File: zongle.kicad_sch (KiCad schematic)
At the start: 20 parts, among them U1 453-00059R

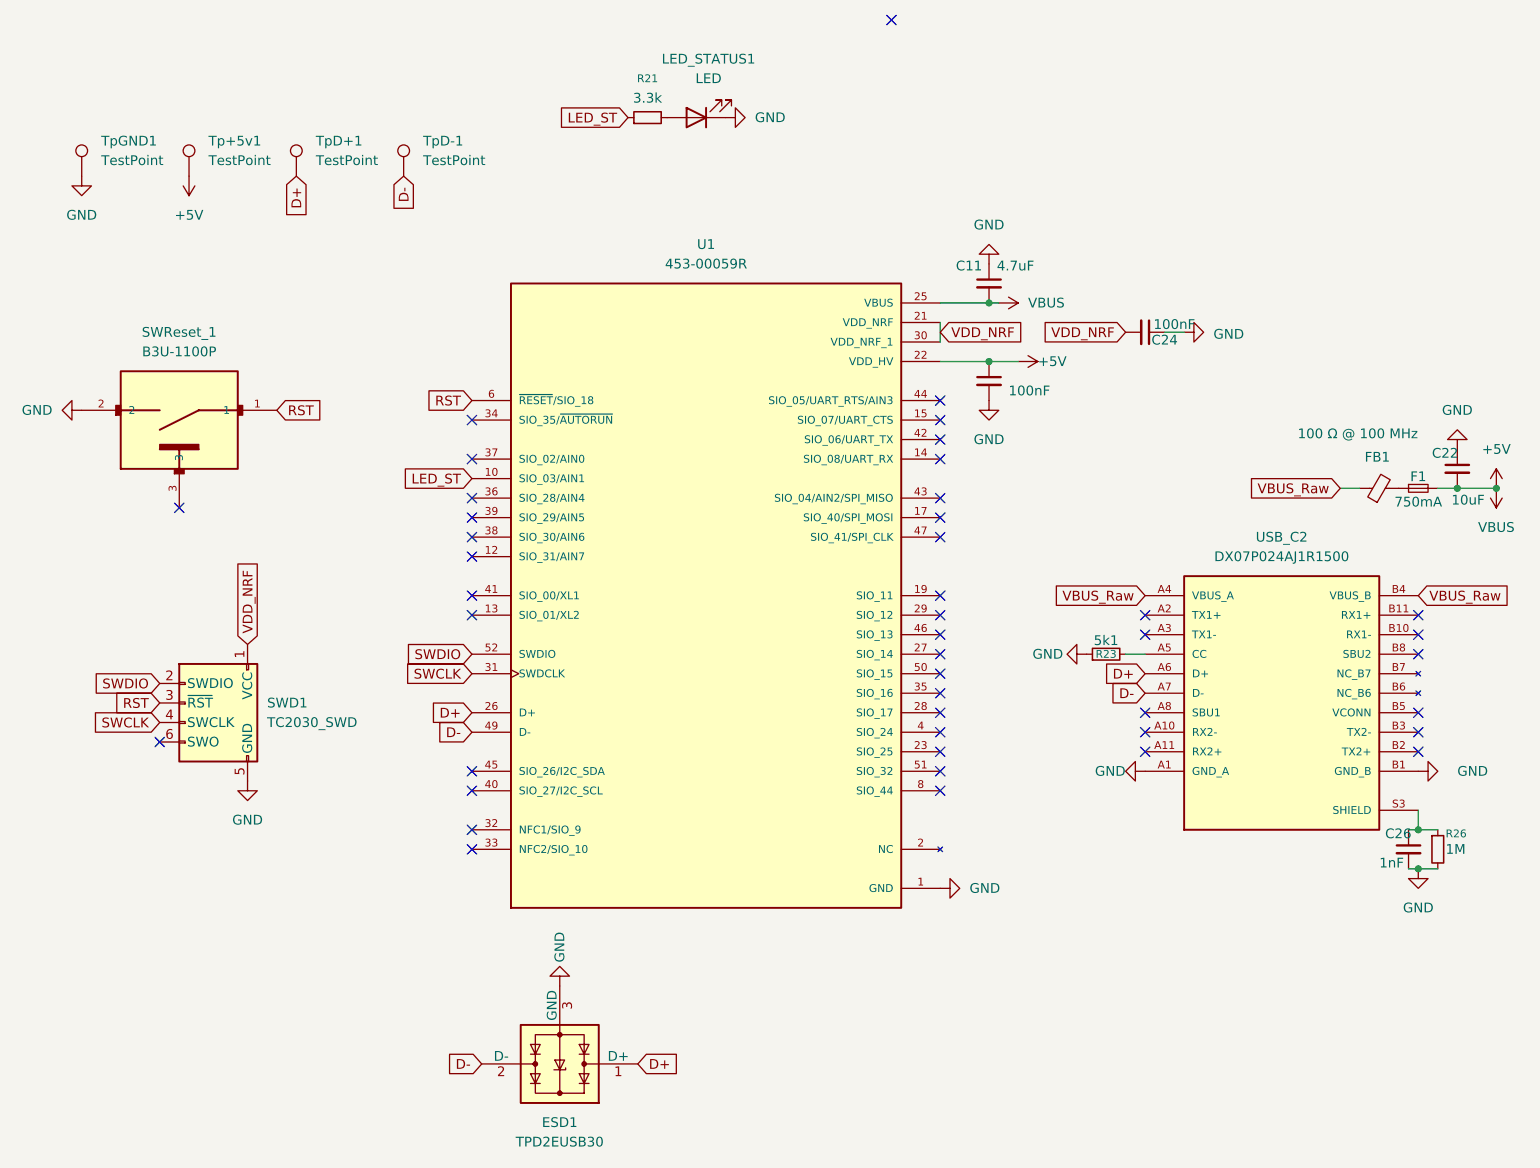
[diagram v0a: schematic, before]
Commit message: minor changes to the routing. final tweaks for first version
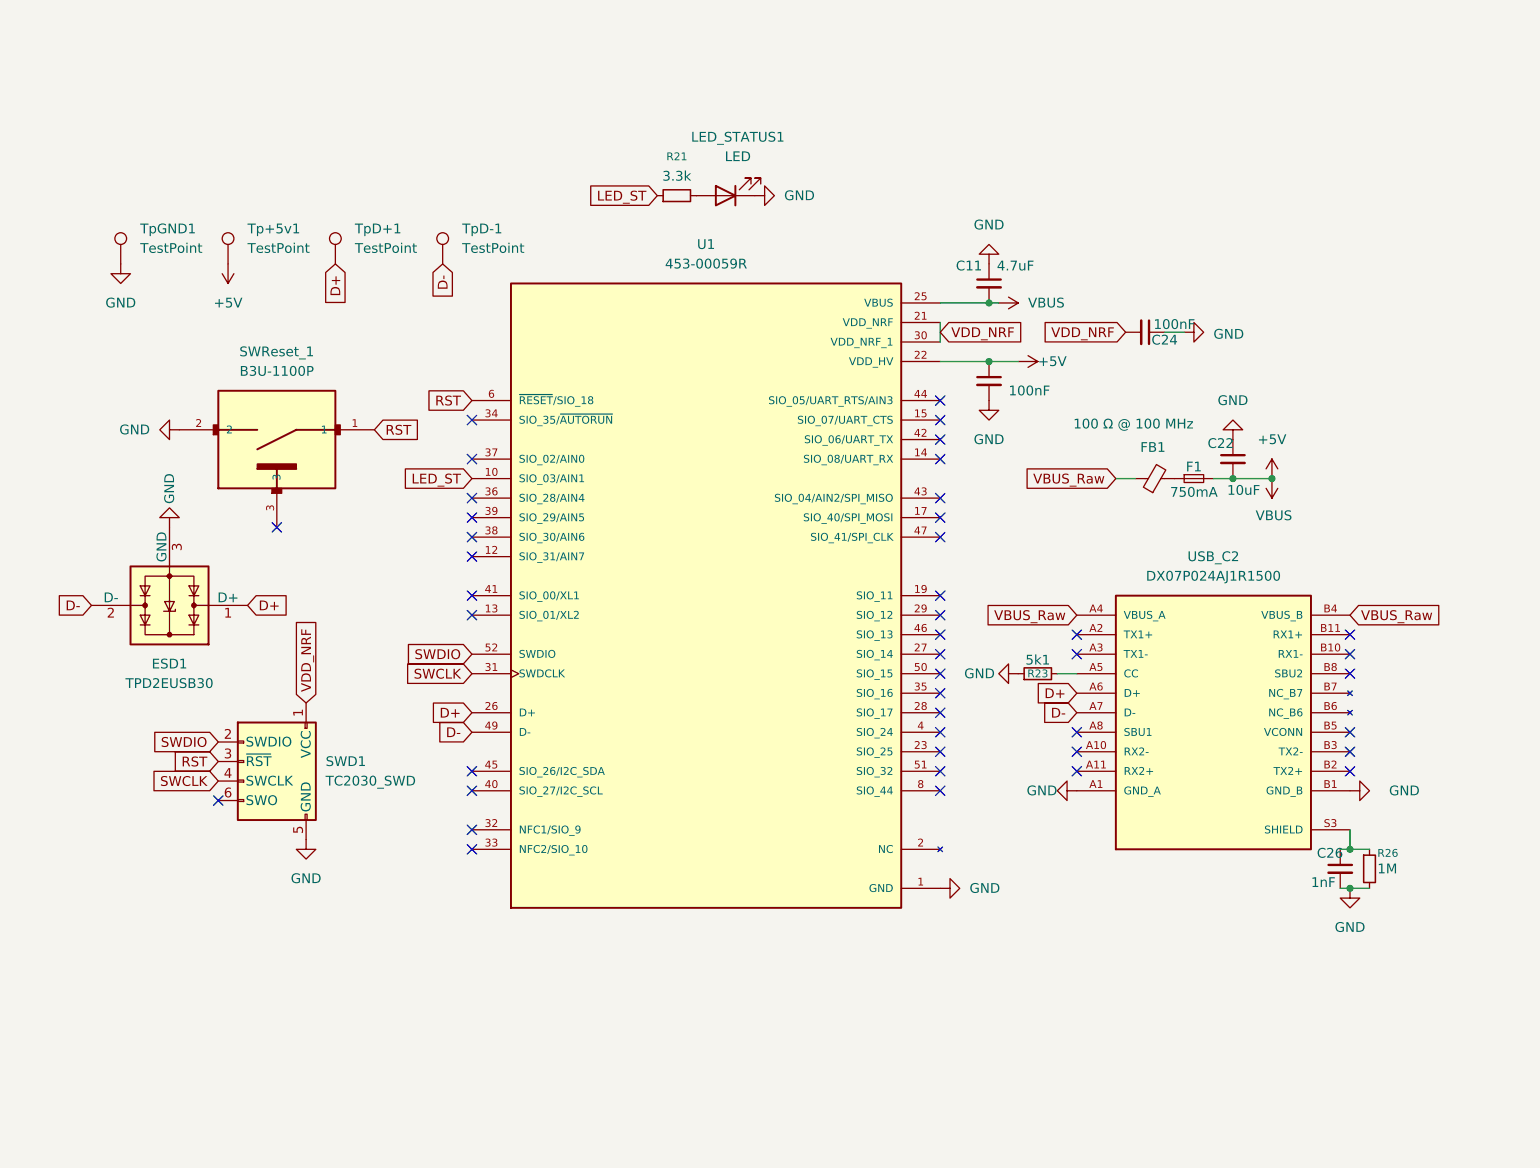
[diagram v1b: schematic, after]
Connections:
- no-connect marks 44 -> 43
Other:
- moved on the sheet: C22, C26, ESD1, F1, FB1, LED_STATUS1, R21, R23, R26, SWD1, SWReset_1, Tp+5v1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
